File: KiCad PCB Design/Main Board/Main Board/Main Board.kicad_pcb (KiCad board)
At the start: 2 copper layers, 19 x 27.9 mm, 7 parts, among them J1 Conn_01x10_Male, J2 Conn_01x10_Male, J3 Conn_01x10_Male, J4 Conn_01x10_Male, U1 ATtiny412-SS

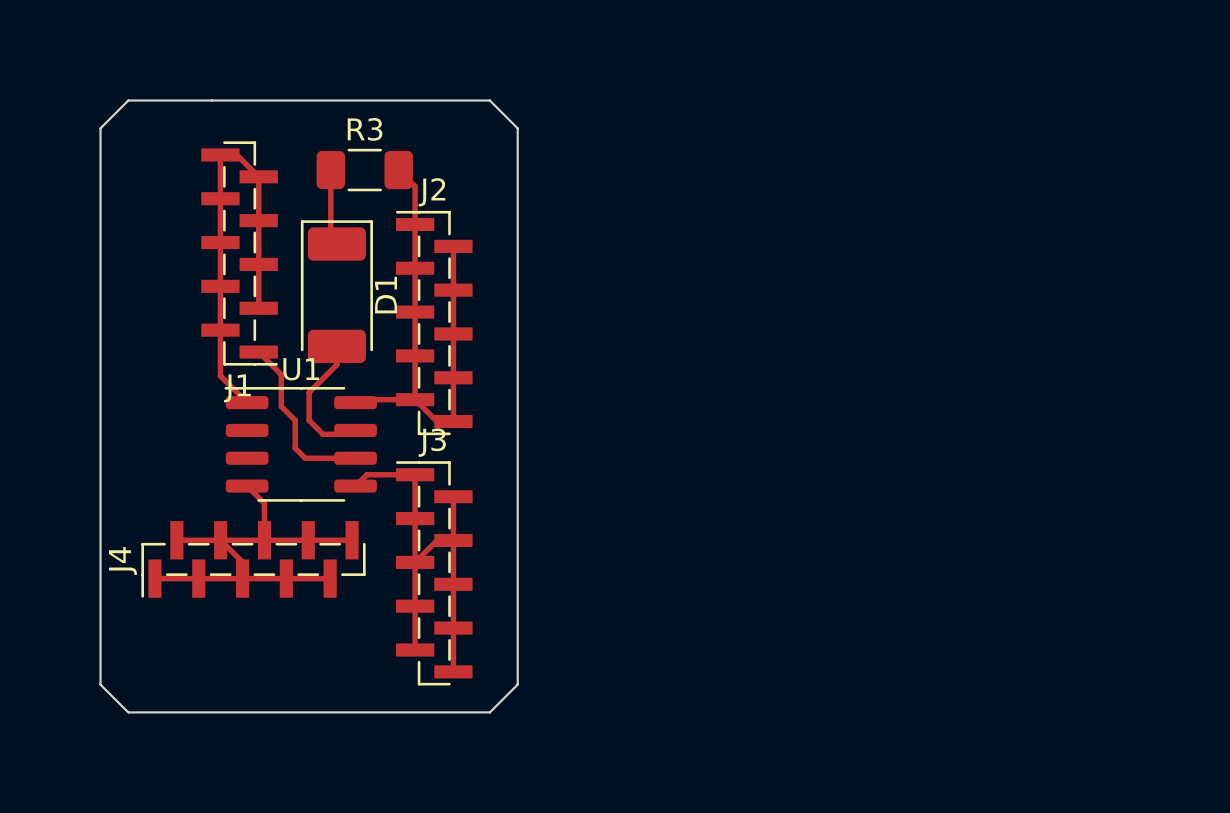
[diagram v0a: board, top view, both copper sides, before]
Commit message: v1.3 - Main PCB Board Updated To Fab Library
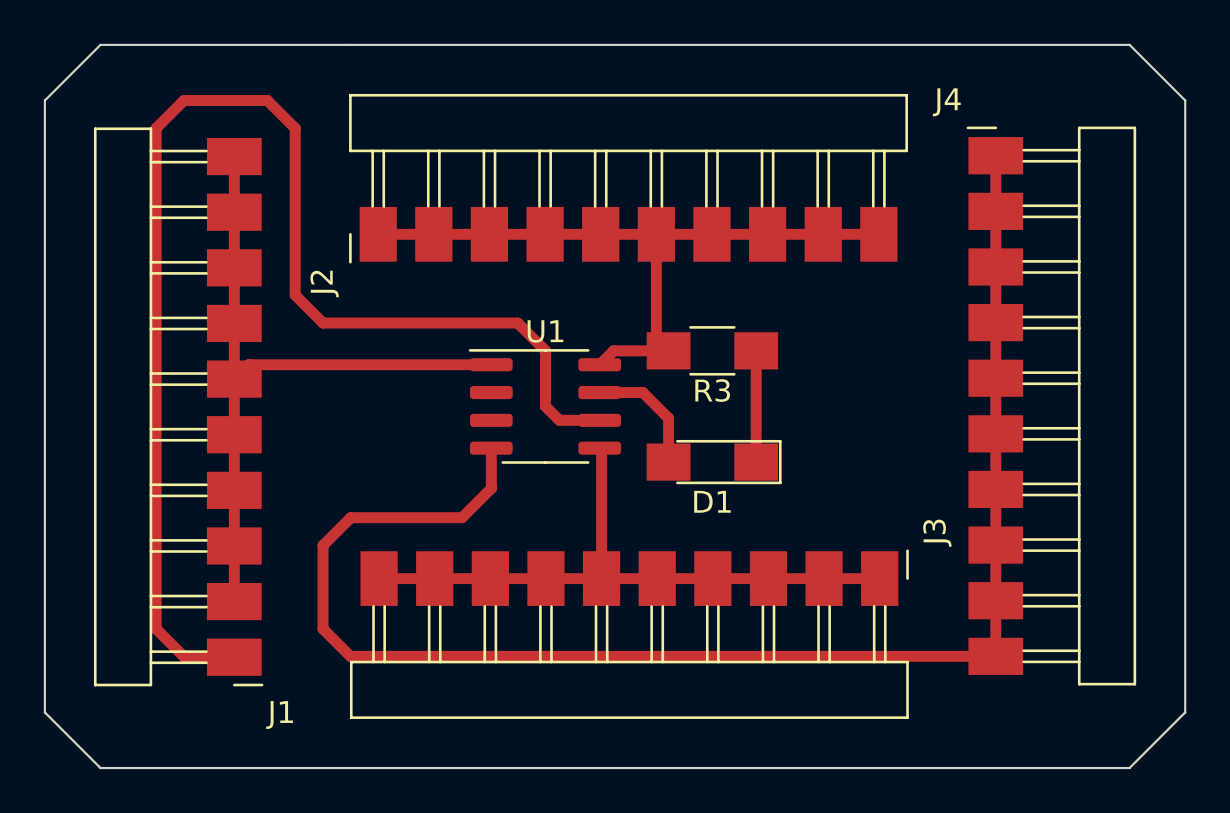
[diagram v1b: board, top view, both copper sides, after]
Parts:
- D1: footprint LED_SMD:LED_2010_5025Metric_Pad1.52x2.65mm_HandSolder -> fab:LED_1206
- J1, J2, J3, J4: footprint Connector_PinHeader_1.00mm:PinHeader_1x10_P1.00mm_Vertical_SMD_Pin1Left -> fab:PinHeader_1x10_P2.54mm_Horizontal_SMD
- R3: footprint Resistor_SMD:R_1206_3216Metric_Pad1.30x1.75mm_HandSolder -> fab:R_1206
- moved J4 38.6 mm to (197.1, 80.0), turned to 0 degrees
- moved J3 20.3 mm to (191.8, 99.3), turned to -90 degrees
- moved D1 18.8 mm to (184.2, 94.0), turned to 180 degrees
- moved J1 18.4 mm to (162.3, 102.9)
- moved R3 17.9 mm to (184.2, 88.9), turned to 180 degrees
- moved U1 11.3 mm to (176.5, 91.4)
- moved J2 4.79 mm to (168.9, 83.6), turned to 90 degrees
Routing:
- net Net-(J1-Pad1): track 8.03 -> 59.7 mm
- net Net-(J4-Pad1): track 21.0 -> 68.5 mm
- net Net-(J1-Pad10): track 20.0 -> 32.3 mm
- net Net-(J2-Pad1): track 23.7 -> 31.8 mm
- net Net-(J3-Pad1): track 21.1 -> 28.9 mm
- net Net-(D1-Pad1): track 3.49 -> 5.08 mm
- net Net-(D1-Pad2): track 6.36 -> 5.63 mm
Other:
- board size 19 x 27.9 mm -> 52.1 x 33 mm
